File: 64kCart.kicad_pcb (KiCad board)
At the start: 2 copper layers, 58.2 x 62.1 mm, 10 parts, among them SW1 SW_Push, U1 27C512, U2 74LS173, U3 74LS04, U4 C64-Exp-Port

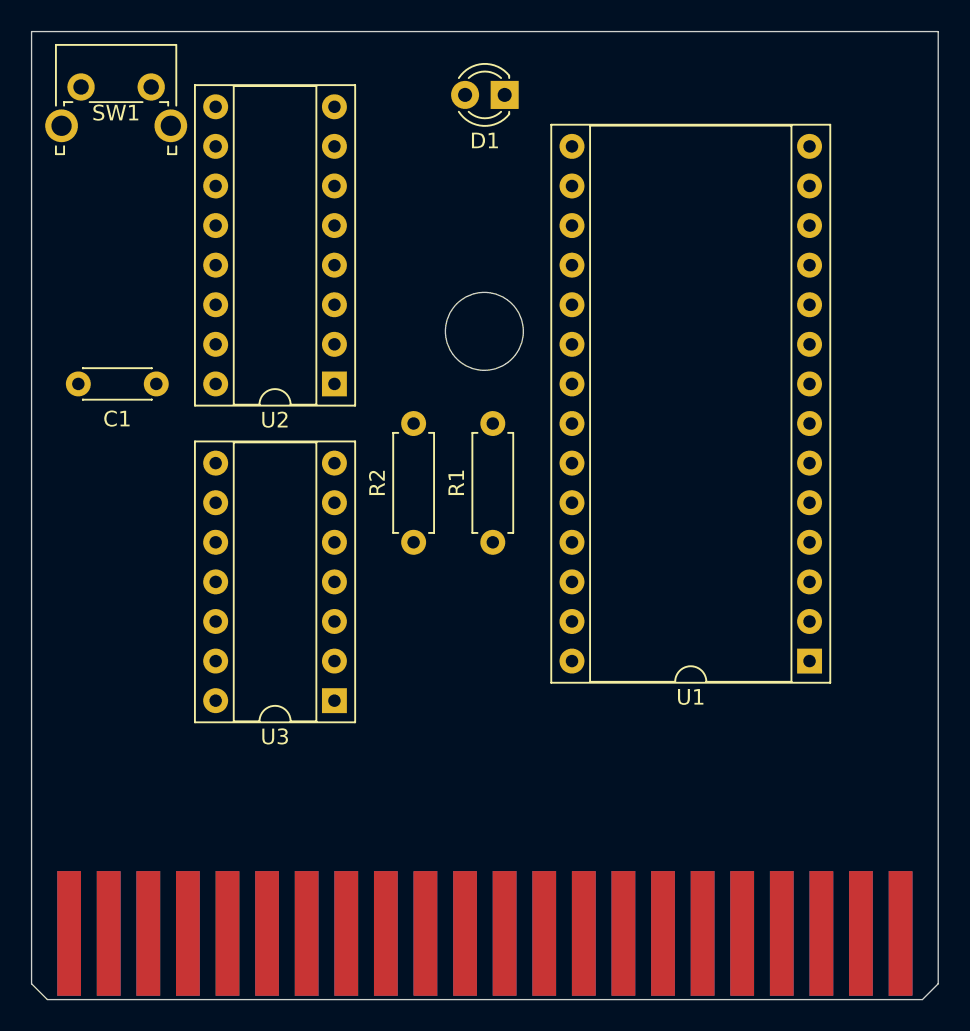
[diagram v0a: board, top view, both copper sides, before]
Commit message: First layout completed.
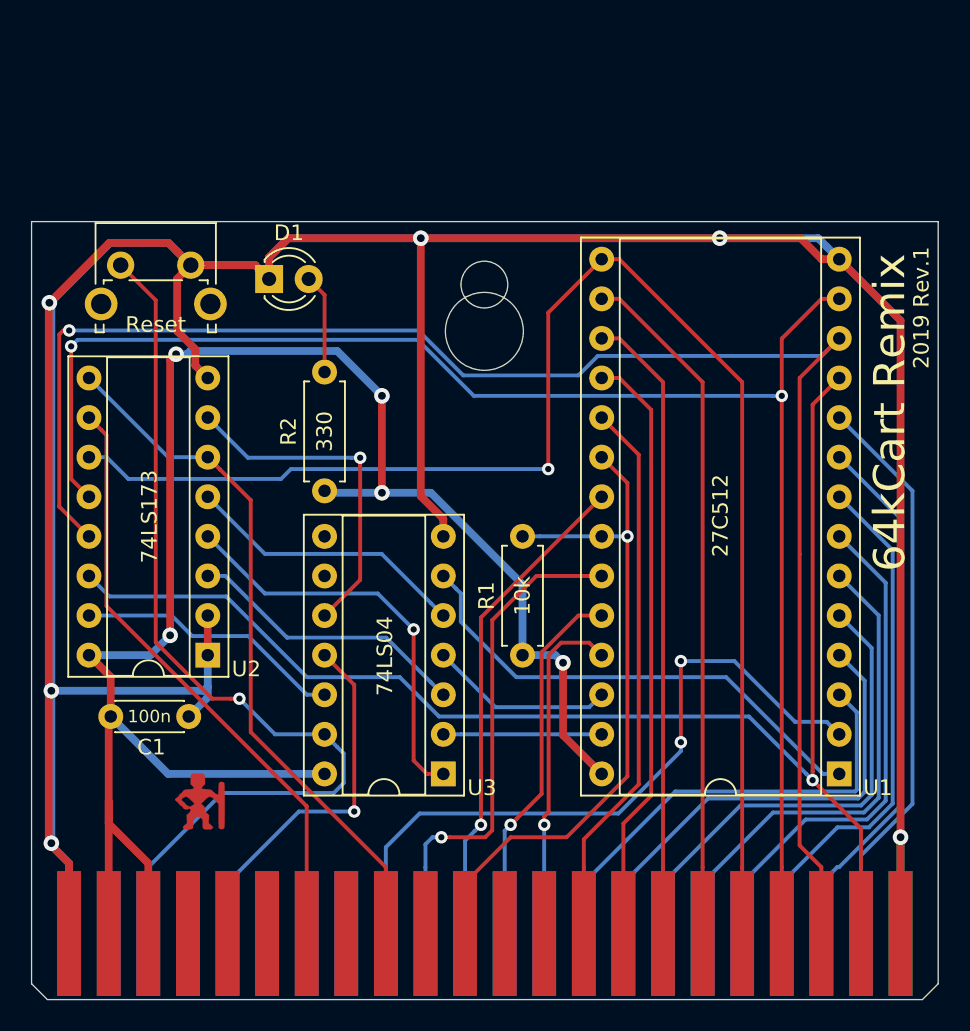
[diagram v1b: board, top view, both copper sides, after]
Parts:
- added G***: LOGO, Logo:bigby2, F.Cu at (118.7, 126.0)
- H1: footprint Mounting_Holes:MountingHole_5mm -> 64kCart:MountingHole_CartCombined
- SW1: value SW_Push -> Reset
- moved C1 21.5 mm to (112.9, 120.7), turned to 0 degrees
- moved U2 19.2 mm to (119.1, 116.7)
- moved D1 19.2 mm to (123.1, 92.6), turned to 0 degrees
- moved SW1 11.7 mm to (113.5, 91.7)
- moved U3 8.42 mm to (134.2, 124.3)
- moved U1 7.49 mm to (159.6, 124.3)
- moved R1 7.49 mm to (139.3, 116.7)
- moved R2 6.60 mm to (126.6, 106.2)
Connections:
- U4 pad 10: Net-(U4-Pad10) -> (no net)
- U4 pad 12: Net-(U4-Pad12) -> (no net)
- U4 pad 13: Net-(U4-Pad13) -> (no net)
- U4 pad 4: Net-(U4-Pad4) -> (no net)
- U4 pad 5: Net-(U4-Pad5) -> (no net)
- U4 pad 6: Net-(U4-Pad6) -> (no net)
- U4 pad 8: Net-(U4-Pad8) -> (no net)
- U4 pad B: Net-(U4-PadB) -> (no net)
- U4 pad D: Net-(U4-PadD) -> (no net)
- U4 pad F: Net-(U4-PadF) -> (no net)
- U4 pad H: Net-(U4-PadH) -> (no net)
- U4 pad J: Net-(U4-PadJ) -> (no net)
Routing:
- net GND: track 0.00 -> 289.6 mm, vias 0 -> 6
- net +5V: track 0.00 -> 118.6 mm, vias 0 -> 5
- net /D1: track 0.00 -> 105.9 mm, vias 0 -> 1
- net /D2: track 0.00 -> 100.3 mm, vias 0 -> 2
- net /D3: track 0.00 -> 92.8 mm, vias 0 -> 1
- net /D0: track 0.00 -> 89.5 mm, vias 0 -> 1
- net /RESET: track 0.00 -> 61.1 mm, vias 0 -> 1
- net /EXROM: track 0.00 -> 45.0 mm
- net /A12: track 0.00 -> 44.9 mm, vias 0 -> 2
- net /ROML: track 0.00 -> 44.4 mm, vias 0 -> 1
- net /D4: track 0.00 -> 44.1 mm
- net /D5: track 0.00 -> 40.5 mm
- net /IO1: track 0.00 -> 38.9 mm
- net /D6: track 0.00 -> 38.3 mm
- net /A0: track 0.00 -> 36.4 mm
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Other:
- board size 58.2 x 62.1 mm -> 58.2 x 49.9 mm
- net class Power: trace_width 0.4 -> 0.5
- board text added: "2019 Rev.1"
- board text added: "64kCart Remix"
- board text added: "64kCart Remix 2019 Rev.1 - https://www.hackup.net Based on the original "64k Karte" design by Hucky."
